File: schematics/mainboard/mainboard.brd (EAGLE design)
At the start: 183 x 105 mm, 144 parts, among them IC1 LM358N, IC2 LM339N, IC3 74AHC00D, IC4 LM2576-5.0, IC5 LM2576-3.3, Q1 BD140, Q2 BD140, Q3 IRL520, T1 2N3904, T2 2N3904, T3 BC847, T4 BC847, T5 BC847, T6 BC847, T7 BC847, T8 BC847, U1 STM32F777VIT, X1 SUPPLY

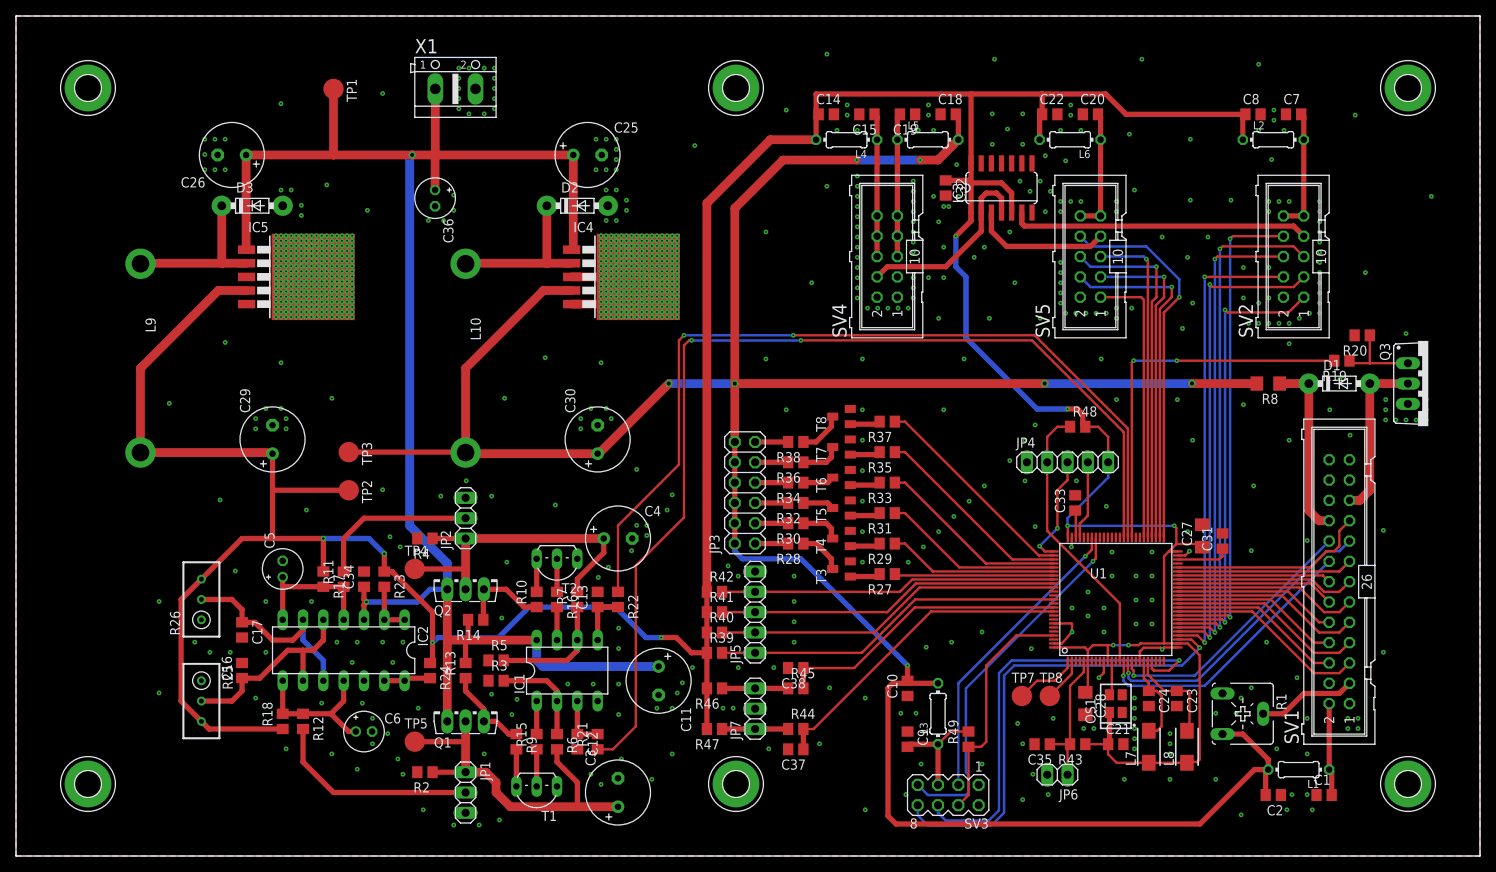
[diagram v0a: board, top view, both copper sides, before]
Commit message: Add files via upload
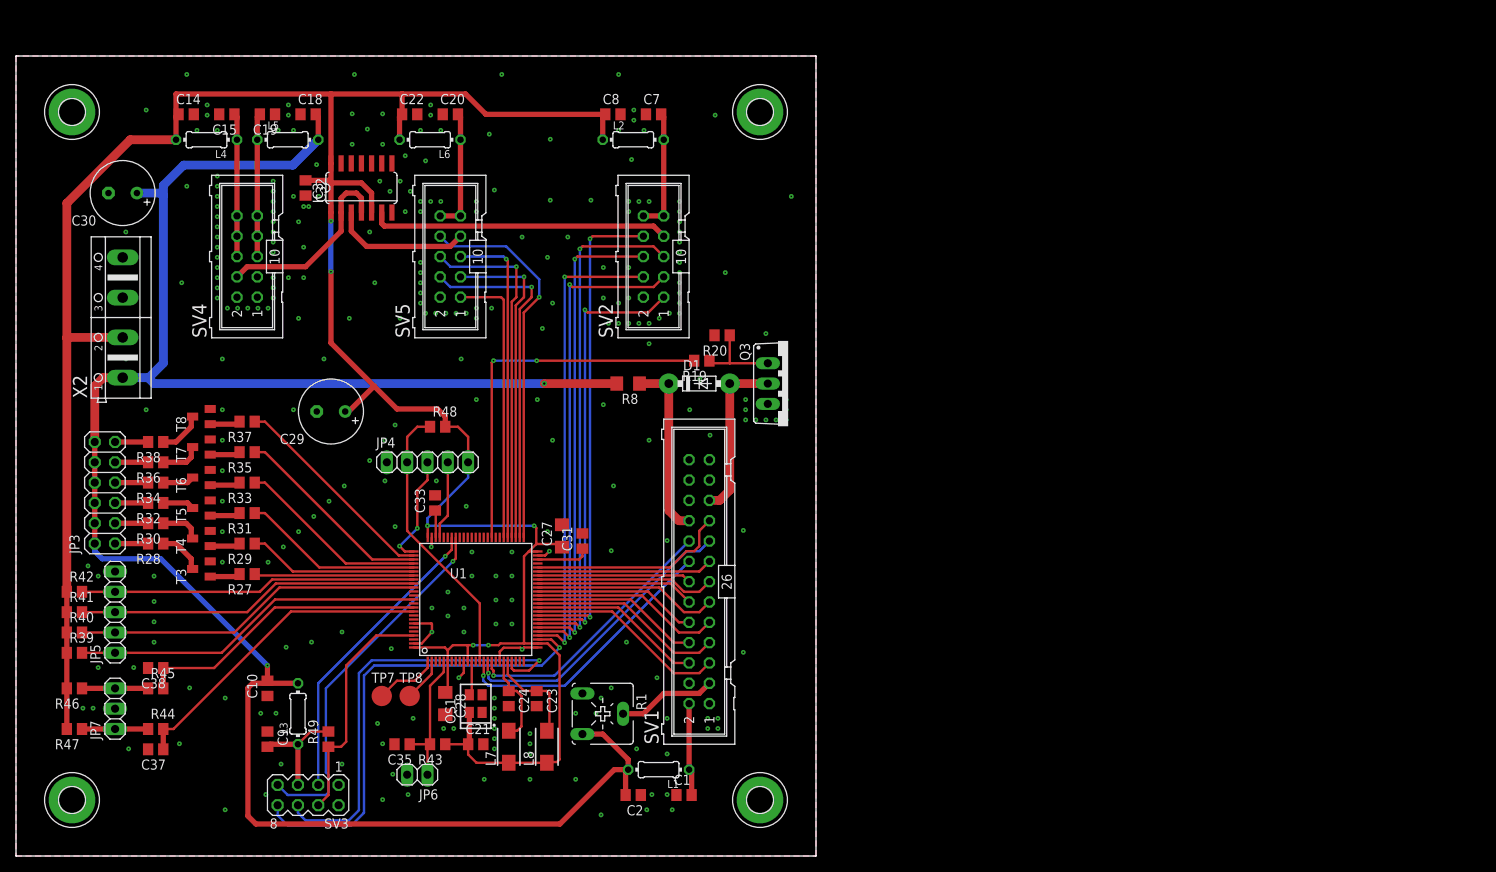
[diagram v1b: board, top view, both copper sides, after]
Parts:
- removed C11, C25, C26, C3, C4: 100u/35V, rcl:E3,5-8
- removed C12, C13: 1u, rcl:C0805
- removed C16, C17: 100n, rcl:C0805
- removed C34: 4.7u, rcl:C0805
- removed C36, C5, C6: 22u/25, rcl:E2-5
- removed D2, D3: 1N5822, diode:DO41-7.6
- removed H1, H4: MOUNT-PAD-ROUND3.2, holes:3,2-PAD
- removed IC1: LM358N, linear:DIL08
- removed IC2: LM339N, linear:DIL14
- removed IC4: LM2576-5.0, v-reg-3:TO263-5
- removed IC5: LM2576-3.3, v-reg-3:TO263-5
- removed JP1: FAN_R, pinhead:1X03
- removed JP2: FAN_L, pinhead:1X03
- removed L10, L9: 1410454C, rcl:TJ5-U2
- removed Q1, Q2: BD140, transistor-power:TO126AV
- removed R10, R9: 470R, resistor:R0805
- removed R11, R12, R15, R16, R23, R24: 4k7, resistor:R0805
- removed R13, R14, R2, R4: 10k, resistor:R0805
- removed R17, R18, R6, R7: 2k7, resistor:R0805
- removed R21, R22: 22k, resistor:R0805
- removed R25, R26: 10k, rcl:RTRIM3296W
- removed R3, R5: 1k, resistor:R0805
- removed T1, T2: 2N3904, transistor-neu-to92:TO92-EBC
- removed TP1, TP2, TP3, TP4, TP5: TPB2,54, testpad:B2,54
- removed X1: SUPPLY, con-ptr500:AK500/2
- added X2: (no value), con-ptr500:AK500/4
- D1: value 1N5822 -> UF4007
- moved H5 83.1 mm to (7.00, 93.0)
- moved H6 83.0 mm to (7.00, 7.00)
- moved H3 81.1 mm to (93.0, 93.0)
- moved H2 81.0 mm to (93.0, 7.00)
- moved C20 80.0 mm to (54.3, 92.7)
- moved C35 80.0 mm to (48.3, 14.0)
- moved JP6 80.0 mm to (50.2, 10.2)
- moved R19 80.0 mm to (85.7, 61.9)
- moved SV5 80.0 mm to (54.3, 74.9)
- moved C27 80.0 mm to (68.3, 40.0)
- moved C31 80.0 mm to (70.8, 39.4)
- moved C33 80.0 mm to (52.4, 44.1)
- moved C8 80.0 mm to (74.6, 92.7)
- moved JP3 80.0 mm to (11.1, 45.4)
- moved L1 80.0 mm to (80.3, 10.8)
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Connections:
- removed net +12V: C11.+, C25.+, C26.+, C34.1, C36.+, IC1.8, IC2.3, IC4.1, IC5.1, Q1.E, Q2.E, R13.2, R14.2, TP1.TP, X1.1
- removed net L_FAN_OK: IC2.1, IC2.2, R23.2
- removed net N$1: D2.C, IC4.2, L10.1
- removed net N$10: R9.2, T1.C
- removed net N$11: C13.1, IC1.5, R22.2
- removed net N$12: Q1.B, R13.1, R9.1
- removed net N$14: R10.2, T2.C
- removed net N$15: C3.+, JP1.1, Q1.C, R2.1, R6.2, TP5.TP
- removed net N$16: IC1.6, R5.2, R7.1
- removed net N$17: Q2.B, R10.1, R14.1
- removed net N$18: R15.1, T1.B
- removed net N$19: C4.+, JP2.1, Q2.C, R4.1, R7.2, TP4.TP
- removed net N$20: IC1.2, R3.2, R6.1
- removed net N$21: IC1.1, R15.2
- removed net N$22: R16.1, T2.B
- removed net N$23: IC1.7, R16.2
- removed net N$26: C6.+, IC2.11, IC2.8, R12.1, R18.2
- removed net N$27: C5.+, IC2.4, IC2.7, R11.1, R17.2
- removed net N$3: D3.C, IC5.2, L9.1
- removed net N$9: C12.1, IC1.3, R21.2
- removed net R_FAN_OK: IC2.13, IC2.14, R24.2
- removed net TACHO_FAN_L: JP2.2, R11.2
- removed net TACHO_FAN_R: JP1.2, R12.2
- removed net V_DN: C17.1, IC2.10, IC2.6, R26.2
- removed net V_UP: C16.1, IC2.5, IC2.9, R25.2
- net +3V3: now also X2.2; no longer IC5.4, L9.2, R17.1, R18.1, R23.1, R24.1, R25.3, R26.3, TP2.TP
- net +5V: now also X2.1; no longer IC4.4, L10.2, TP3.TP
- net GND: now also X2.3, X2.4; no longer C11.-, C12.2, C13.2, C16.2, C17.2, C25.-, C26.-, C3.-, C34.2, C36.-, C4.-, C5.-, C6.-, D2.A, D3.A, H1.B3,2, H4.B3,2, IC1.4, IC2.12, IC4.3, IC4.5, IC4.6, IC5.3, IC5.5, IC5.6, JP1.3, JP2.3, R2.2, R25.1, R26.1, R3.1, R4.2, R5.1, T1.E, T2.E, X1.2
- net PWM_FAN_L: no longer R22.1
- net PWM_FAN_R: no longer R21.1
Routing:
- net +12V: track 208.4 -> 0.00 mm, vias 2 -> 0
- net +3V3: track 509.3 -> 339.5 mm, vias 10 -> 6
- net PWM_FAN_R: track 129.2 -> 0.00 mm, vias 2 -> 0
- net PWM_FAN_L: track 109.4 -> 0.00 mm, vias 2 -> 0
- net +5V: track 337.4 -> 254.7 mm, vias 7 -> 2
- net N$15: track 46.6 -> 0.00 mm
- net N$19: track 42.1 -> 0.00 mm
- net V_DN: track 26.2 -> 0.00 mm
- net TACHO_FAN_R: track 26.0 -> 0.00 mm
- net V_UP: track 25.7 -> 0.00 mm
- net N$1: track 20.5 -> 0.00 mm
- net N$3: track 20.5 -> 0.00 mm
- net TACHO_FAN_L: track 20.4 -> 0.00 mm
- net N$26: track 19.0 -> 0.00 mm
- net GND: track 36.0 -> 17.8 mm, vias 954 -> 271
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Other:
- board size 183 x 105 mm -> 100 x 100 mm
- board text removed: "+12V"
- board text removed: "+3.3V"
- board text removed: "+5V"
- board text removed: "FAN_L"
- board text removed: "FAN_R"
- board text removed: "LEFT"
- board text removed: "RIGHT"
- board text removed: "SUPPLY"
- board text removed: "V_DN"
- board text removed: "V_UP"
